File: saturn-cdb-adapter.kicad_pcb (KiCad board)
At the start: 2 copper layers, 76.2 x 76.2 mm, 60 parts, among them P1 CONN_02X22, P2 CONN_02X20, P3 CONN_02X20, P4 CONN_02X20, P5 CONN_02X20, U1 SH1, U2 MT28EW_FLASH

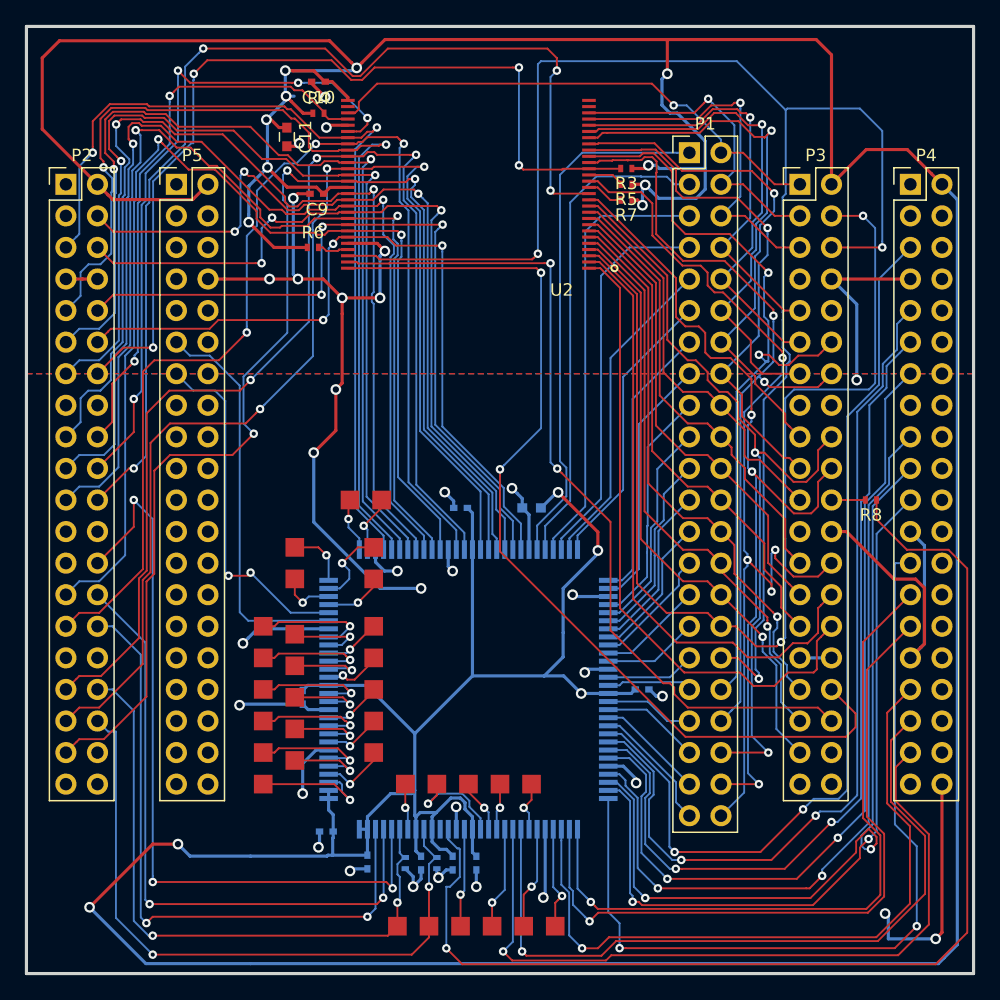
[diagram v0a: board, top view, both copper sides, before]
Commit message: Trace cleanup
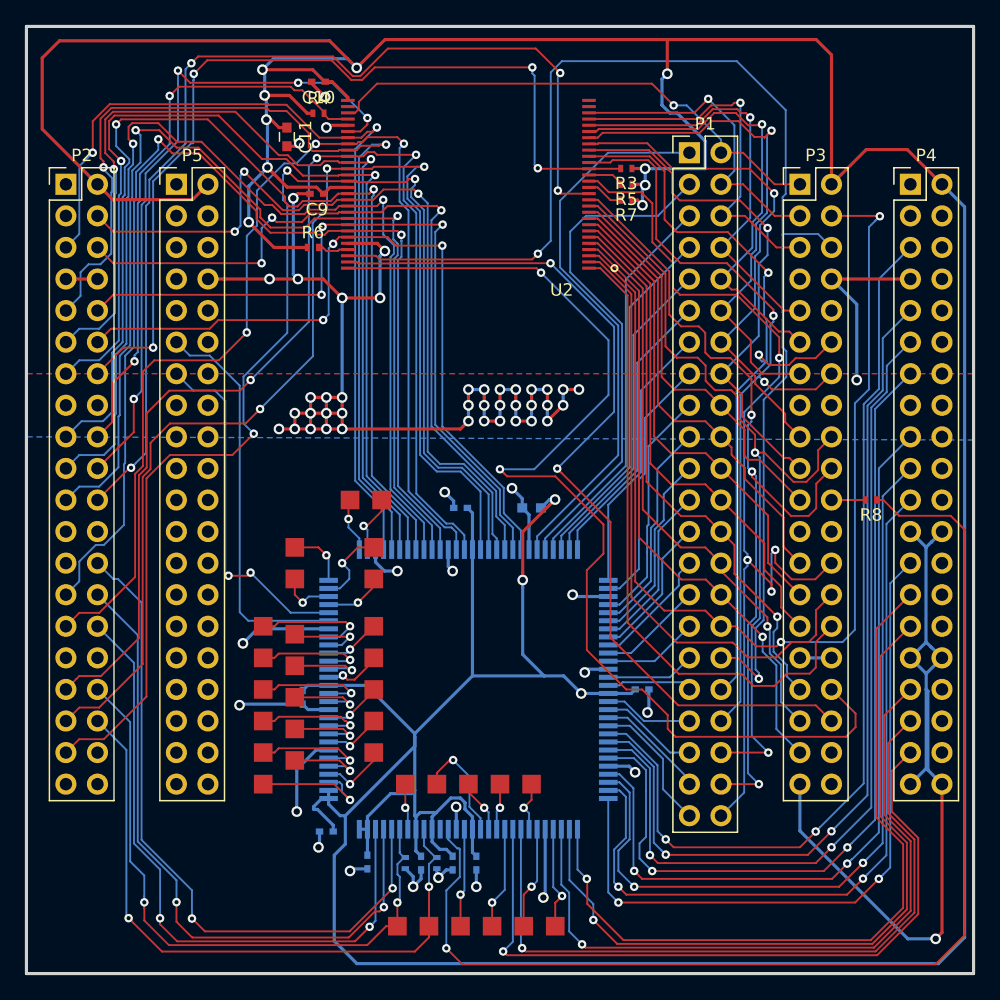
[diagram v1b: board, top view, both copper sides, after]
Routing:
- net GND: track 187.8 -> 246.7 mm, vias 33 -> 62
- net +3V3: track 445.0 -> 417.1 mm, vias 15 -> 13
- net FLASH_A16: track 125.7 -> 106.8 mm, vias 3 -> 2
- net CPU_~CS7: track 68.2 -> 56.9 mm
- net FLASH_A24: track 78.4 -> 89.1 mm
- net MD0: track 62.0 -> 54.8 mm, vias 3 -> 2
- net CPU_~WRL~/~WR: track 56.6 -> 61.2 mm
- net /Flash and CPU/CPU_A2: track 35.6 -> 31.4 mm
- net CPU_~CS5: track 66.7 -> 63.1 mm
- net FLASH_A25: track 69.3 -> 72.8 mm
- net CPU_~WRH~/~LBS~: track 56.4 -> 59.9 mm
- net /Flash and CPU/CPU_A3: track 31.4 -> 28.6 mm
- net MD1: track 51.2 -> 53.4 mm
- net /Flash and CPU/CPU_A0: track 42.5 -> 44.7 mm
- net ~FLASH_WE: track 84.7 -> 82.8 mm
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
